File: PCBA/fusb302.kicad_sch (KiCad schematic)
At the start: 3 parts, among them U301 FUSB302B

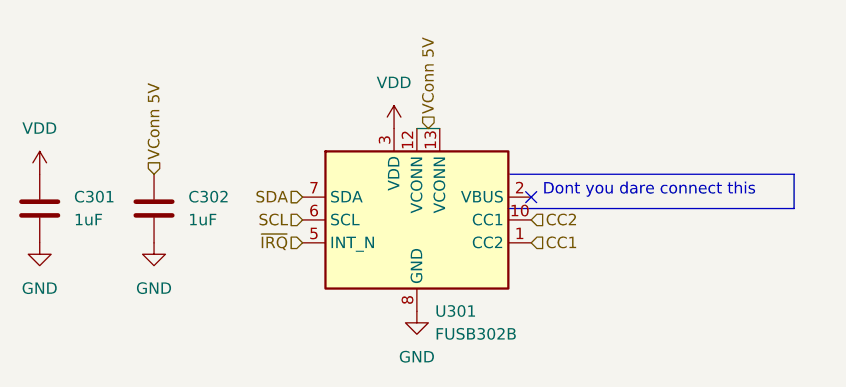
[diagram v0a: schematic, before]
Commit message: Finish routing
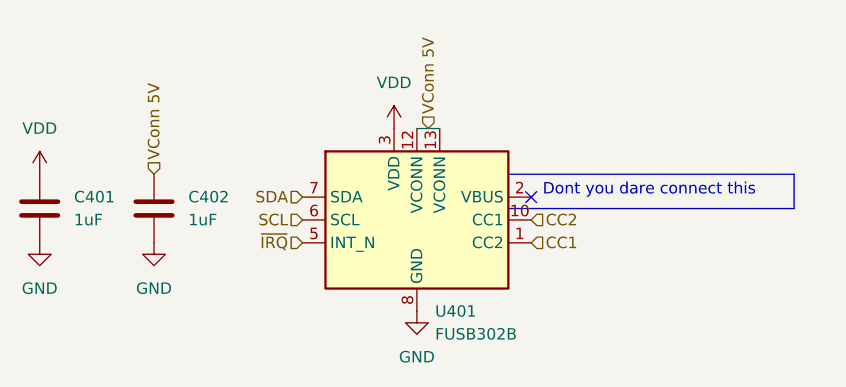
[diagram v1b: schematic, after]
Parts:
- renumbered C301 to C401, C302 to C402, U301 to U401
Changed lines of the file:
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@@
   (symbol (lib_id "Device:C") (at 88.9 85.09 0)
     (in_bom yes) (on_board yes) (fields_autoplaced)
-    (property "Reference" "C301" (id 0) (at 92.71 83.8199 0)
+    (property "Reference" "C401" (id 0) (at 92.71 83.8199 0)
       (effects (font (size 1.27 1.27)) (justify left))
     )
@@
   (symbol (lib_id "Device:C") (at 101.6 85.09 0)
     (in_bom yes) (on_board yes) (fields_autoplaced)
-    (property "Reference" "C302" (id 0) (at 105.41 83.8199 0)
+    (property "Reference" "C402" (id 0) (at 105.41 83.8199 0)
       (effects (font (size 1.27 1.27)) (justify left))
     )
@@
   (symbol (lib_id "Interface_USB:FUSB302B01MPX") (at 130.81 86.36 0)
     (in_bom yes) (on_board yes) (fields_autoplaced)
-    (property "Reference" "U301" (id 0) (at 132.8294 96.52 0)
+    (property "Reference" "U401" (id 0) (at 132.8294 96.52 0)
       (effects (font (size 1.27 1.27)) (justify left))
     )
